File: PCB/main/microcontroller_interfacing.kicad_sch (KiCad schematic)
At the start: 18 parts, among them J5 Conn_01x02_Male, U1 USB_Micro_B, U2 CH340G, U3 AT24C256C-SSHL-T, X1 12MHz Crystal

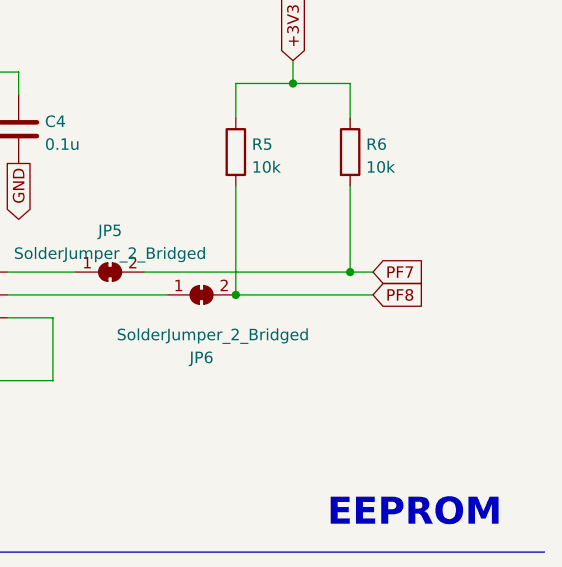
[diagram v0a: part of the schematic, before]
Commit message: Update paths
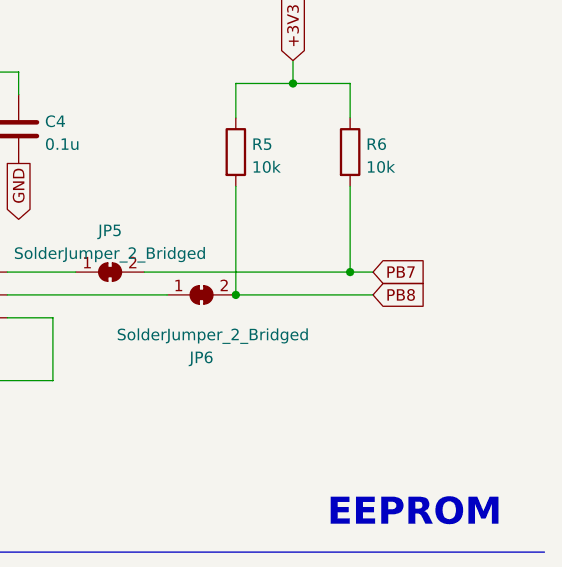
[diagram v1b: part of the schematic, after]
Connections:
- net PF7 renamed PB7
- net PF8 renamed PB8
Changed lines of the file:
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@@
     )
   )
-  (global_label "PF8" (shape input) (at 265.43 47.625 0) (fields_autoplaced)
+  (global_label "PB8" (shape input) (at 265.43 47.625 0) (fields_autoplaced)
     (effects (font (size 1.27 1.27)) (justify left))
-    (property "Intersheet References" "${INTERSHEET_REFS}" (id 0) (at 271.4112 47.5456 0)
+    (property "Intersheet References" "${INTERSHEET_REFS}" (id 0) (at 271.5926 47.5456 0)
       (effects (font (size 1.27 1.27)) (justify left) hide)
     )
@@
     )
   )
-  (global_label "PF7" (shape input) (at 265.43 45.085 0) (fields_autoplaced)
+  (global_label "PB7" (shape input) (at 265.43 45.085 0) (fields_autoplaced)
     (effects (font (size 1.27 1.27)) (justify left))
-    (property "Intersheet References" "${INTERSHEET_REFS}" (id 0) (at 271.4112 45.0056 0)
+    (property "Intersheet References" "${INTERSHEET_REFS}" (id 0) (at 271.5926 45.0056 0)
       (effects (font (size 1.27 1.27)) (justify left) hide)
     )

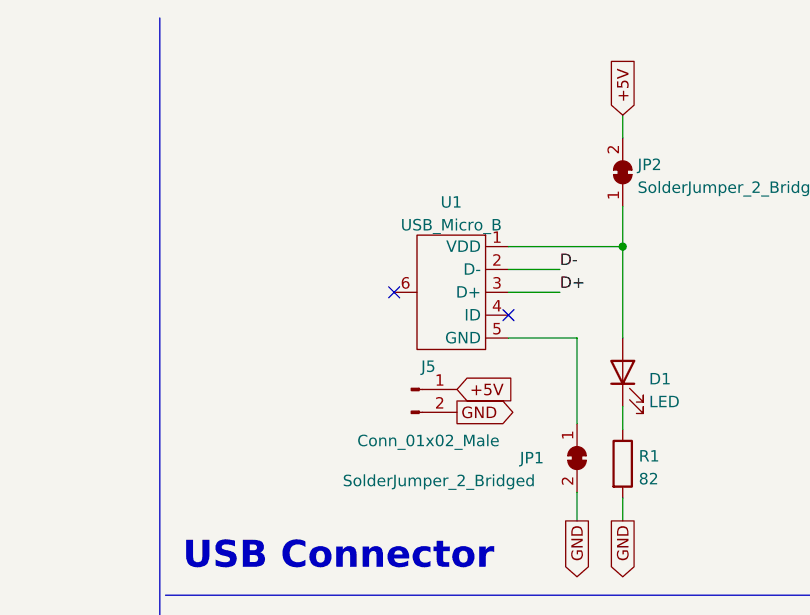
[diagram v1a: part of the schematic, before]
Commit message: Change ports
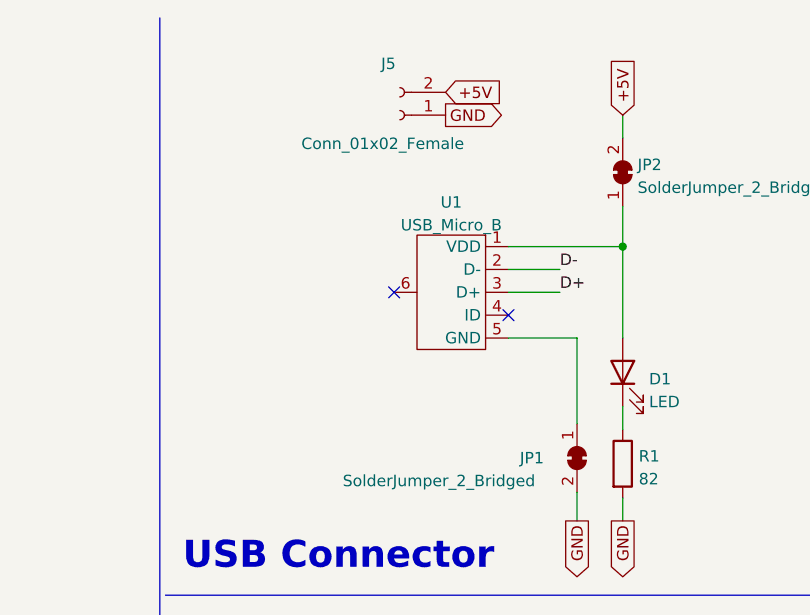
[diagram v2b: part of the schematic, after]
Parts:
- removed J5: Conn_01x02_Male, Connector_PinHeader_1.00mm:PinHeader_1x02_P1.00mm_Vertical, symbol Connector:Conn_01x02_Male
- added J5: Conn_01x02_Female, symbol Connector:Conn_01x02_Female
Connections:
- net +5V: now also J5.2 (Pin_2)
- net GND: now also J5.1 (Pin_1)
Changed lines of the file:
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@@
     )
   )
-  (global_label "+5V" (shape input) (at 141.605 53.34 0) (fields_autoplaced)
+  (global_label "+5V" (shape input) (at 140.335 20.32 0) (fields_autoplaced)
     (effects (font (size 1.27 1.27)) (justify left))
-    (property "Intersheet References" "${INTERSHEET_REFS}" (id 0) (at 147.8886 53.2606 0)
+    (property "Intersheet References" "${INTERSHEET_REFS}" (id 0) (at 146.6186 20.2406 0)
       (effects (font (size 1.27 1.27)) (justify left) hide)
     )
   )
-  (global_label "GND" (shape output) (at 141.605 55.88 0) (fields_autoplaced)
+  (global_label "GND" (shape output) (at 140.335 22.86 0) (fields_autoplaced)
     (effects (font (size 1.27 1.27)) (justify left))
-    (property "Intersheet References" "${INTERSHEET_REFS}" (id 0) (at 147.8886 55.8006 0)
+    (property "Intersheet References" "${INTERSHEET_REFS}" (id 0) (at 146.6186 22.7806 0)
       (effects (font (size 1.27 1.27)) (justify left) hide)
     )
@@
     (pin "2")
   )
+  (symbol (lib_id "Connector:Conn_01x02_Female") (at 135.255 22.86 180) (unit 1)
+    (in_bom yes) (on_board yes)
+    (property "Reference" "J5" (id 0) (at 133.985 17.145 0))
+    (property "Value" "Conn_01x02_Female" (id 1) (at 133.35 26.035 0))
+    (property "Footprint" "" (id 2) (at 135.255 22.86 0)
+      (effects (font (size 1.27 1.27)) hide)
+    )
+    (property "Datasheet" "~" (id 3) (at 135.255 22.86 0)
+      (effects (font (size 1.27 1.27)) hide)
+    )
+    (pin "1")
+    (pin "2")
+  )
   (symbol (lib_id "Device:R") (at 160.02 61.595 0) (unit 1)
     (in_bom yes) (on_board yes) (fields_autoplaced)
@@
       (effects (font (size 1.27 1.27)) hide)
     )
-    (pin "1")
-    (pin "2")
-  )
-  (symbol (lib_id "Connector:Conn_01x02_Male") (at 136.525 53.34 0) (unit 1)
-    (in_bom yes) (on_board yes)
-    (property "Reference" "J5" (id 0) (at 138.43 50.8 0))
-    (property "Value" "Conn_01x02_Male" (id 1) (at 138.43 59.055 0))
-    (property "Footprint" "Connector_PinHeader_1.00mm:PinHeader_1x02_P1.00mm_Vertical" (id 2) (at 136.525 53.34 0)
-      (effects (font (size 1.27 1.27)) hide)
-    )
-    (property "Datasheet" "~" (id 3) (at 136.525 53.34 0)
-      (effects (font (size 1.27 1.27)) hide)
-    )
